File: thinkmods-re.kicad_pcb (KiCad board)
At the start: 2 copper layers, 26.7 x 3 mm, 13 parts, among them J1 ExpressCard, J3 Micro_SD_Card, U1 GL823K-HCY04

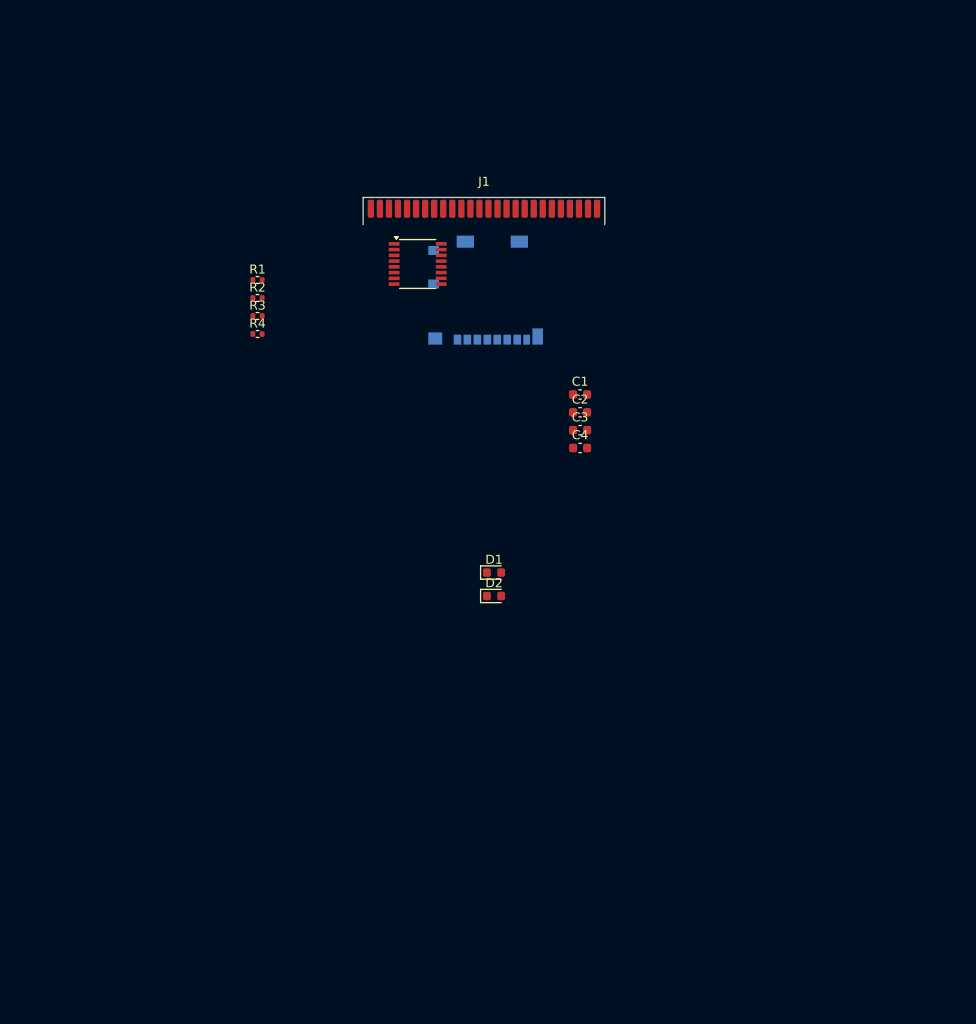
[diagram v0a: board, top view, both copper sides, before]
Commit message: Add files via upload
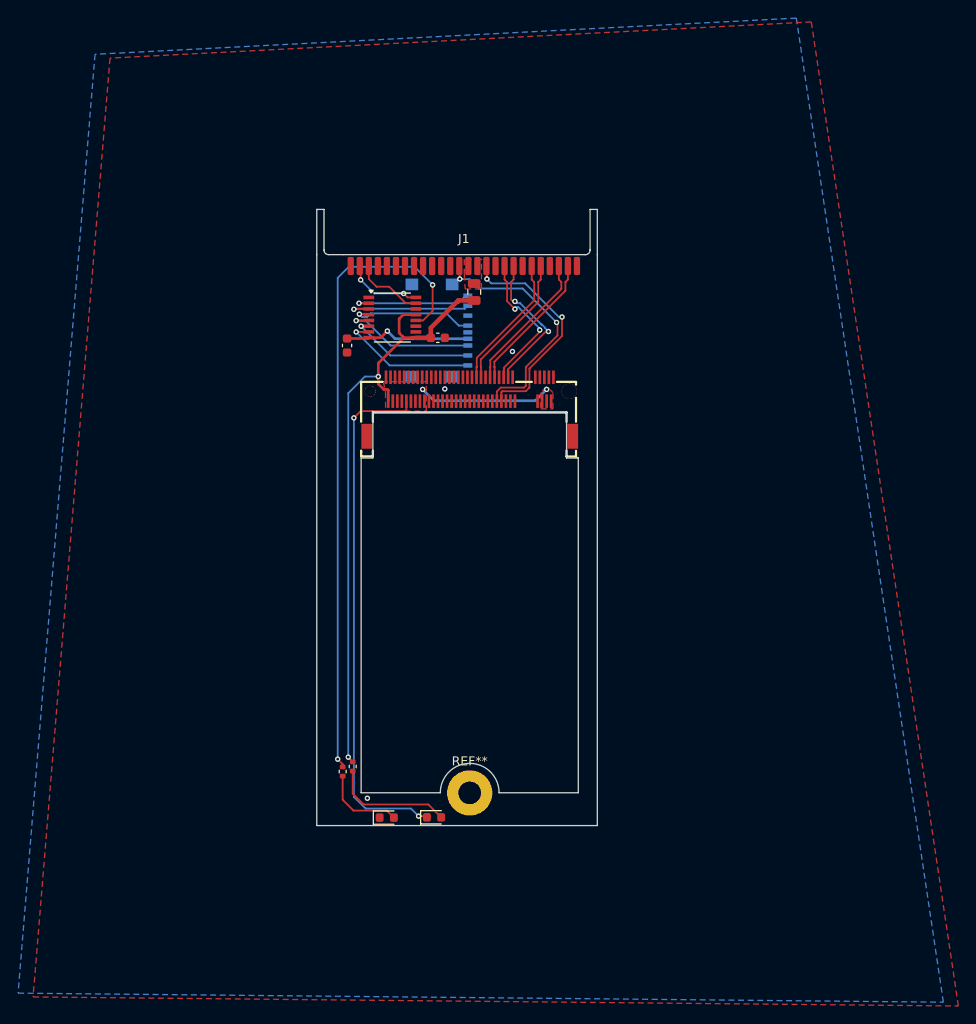
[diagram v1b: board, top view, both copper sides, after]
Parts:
- removed C3, C4: 10uF, Capacitor_SMD:C_0603_1608Metric
- removed R1, R2: 22, Resistor_SMD:R_0402_1005Metric
- added F1: Fuse_Small, Fuse:Fuse_0805_2012Metric, F.Cu at (170.2, 87.1)
- added J2: Bus_M.2_Socket_M, Library:CONN-SMD_APCI0159-P001A, F.Cu at (169.8, 99.8)
- added REF**: MountingHole_2.5mm_Pad, MountingHole:MountingHole_2.5mm_Pad, F.Cu at (169.8, 142.4)
- J3: footprint Connector_Card:microSD_HC_Molex_104031-0811 -> Library:TF-SMD_TF-123-ARP9H15
- moved R3 50.9 mm to (156.8, 139.5), turned to 90 degrees
- moved R4 49.3 mm to (155.7, 140.1), turned to -90 degrees
- moved D1 29.6 mm to (160.6, 145.2)
- moved C1 26.3 mm to (156.2, 93.0), turned to -90 degrees
- moved D2 25.3 mm to (165.8, 145.2)
- moved C2 17.8 mm to (166.2, 92.2)
- moved J3 6.73 mm to (166.4, 91.4), turned to -90 degrees
- moved J1 6.70 mm to (169.1, 84.2)
- moved U1 6.55 mm to (161.2, 89.9)
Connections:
- J1 pad 10: +1V5 -> unconnected-(J1-1V5-Pad10)
- J1 pad 11: /PEWAKE -> unconnected-(J1-~{WAKE}-Pad11)
- J1 pad 14: +3V3 -> /E3V3
- J1 pad 15: +3V3 -> /E3V3
- J1 pad 18: /RCLKn -> /RCLK-
- J1 pad 19: /RCLKp -> /RCLK+
- J1 pad 21: /PCIe_RXn0 -> /PCIe_RX-
- J1 pad 22: /PCIe_RXp0 -> /PCIe_RX+
- J1 pad 24: /PCIe_TXn0 -> /PCIe_TX-
- J1 pad 25: /PCIe_TXp0 -> /PCIe_TX+
- J1 pad 9: +1V5 -> unconnected-(J1-1V5-Pad9)
- U1 pad 15: Net-(U1-DP) -> /USB_D+
- U1 pad 16: Net-(U1-DM) -> /USB_D-
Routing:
- net +3V3: track 0.00 -> 83.2 mm, vias 0 -> 4
- net /SD_LED: track 0.00 -> 71.3 mm, vias 0 -> 2
- net /PCIe_LED: track 0.00 -> 58.0 mm, vias 0 -> 2
- net /PERST: track 0.00 -> 27.1 mm, vias 0 -> 2
- net /CLKREQ: track 0.00 -> 25.1 mm, vias 0 -> 2
- net /RCLK+: track 0.00 -> 16.5 mm, vias 0 -> 2
- net /RCLK-: track 0.00 -> 16.1 mm, vias 0 -> 2
- net /PCIe_TX-: track 0.00 -> 15.7 mm
- net /PCIe_TX+: track 0.00 -> 15.7 mm
- net /SD_DAT2: track 0.00 -> 15.3 mm, vias 0 -> 1
- net /PCIe_RX-: track 0.00 -> 15.1 mm
- net /PCIe_RX+: track 0.00 -> 15.1 mm
- net /SD_CMD: track 0.00 -> 14.9 mm, vias 0 -> 1
- net /SD_DAT0: track 0.00 -> 14.4 mm, vias 0 -> 1
- net /SD_3V3: track 0.00 -> 14.0 mm, vias 0 -> 1
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- added copper zone on F.Cu, net +3V3
- added copper zone on F.Cu, net /E3V3
- added copper zone on B.Cu, net GND
- added copper zone on F.Cu, net GND
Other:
- board size 26.7 x 3 mm -> 31 x 68.1 mm
